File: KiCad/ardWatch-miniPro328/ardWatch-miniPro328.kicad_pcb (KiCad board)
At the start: 2 copper layers, 84.5 x 65.4 mm, 7 parts, among them J1 2-pin_power_input_header, U1 Arduino_Mini_Pro, U2 KY-040_Rotary_Encoder, U3 ST7735_1.8"_TFT_128x160, U4 DS3231_RTC_module

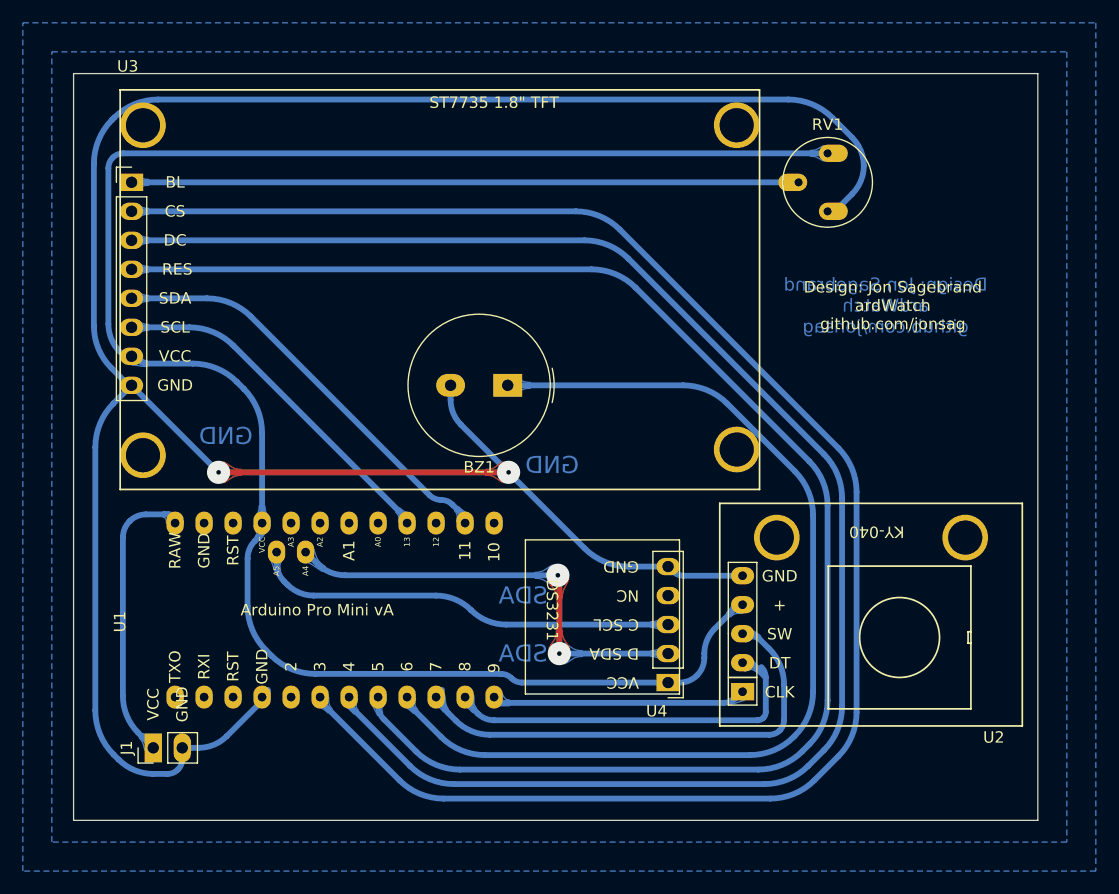
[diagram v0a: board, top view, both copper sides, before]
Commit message: revised pcb
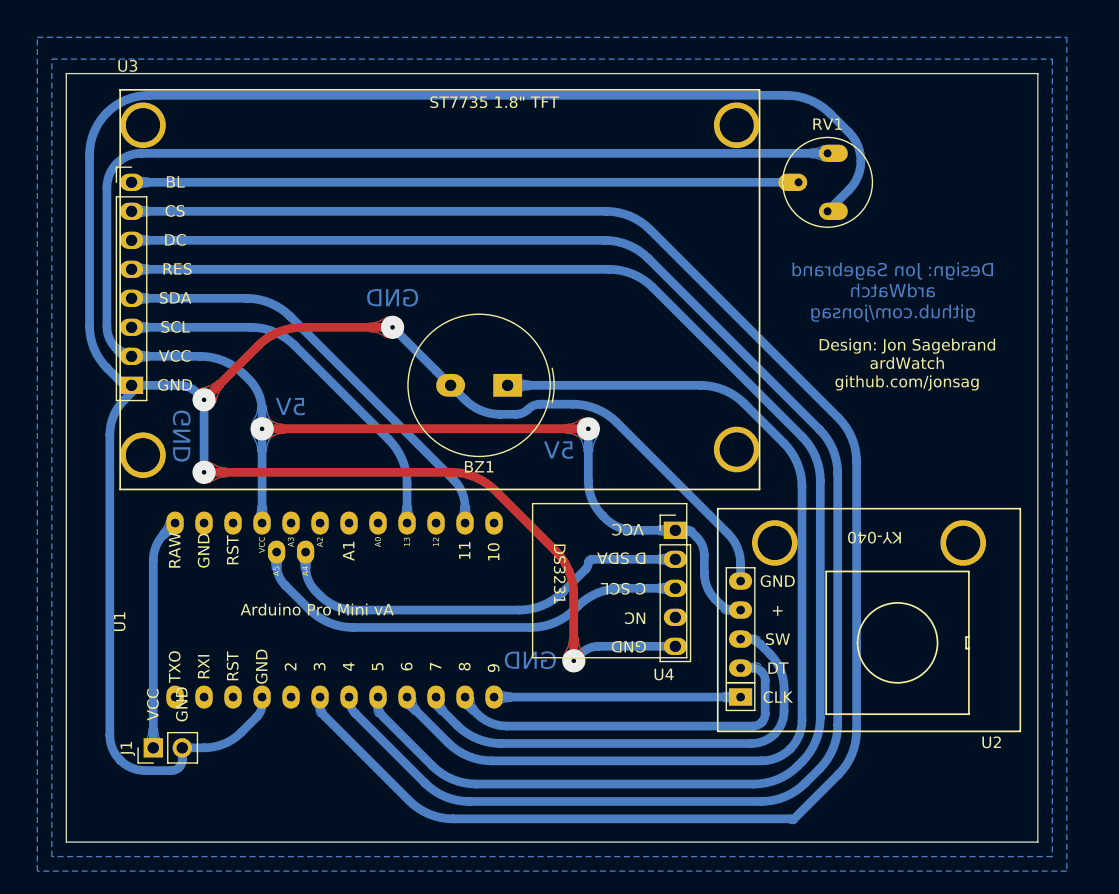
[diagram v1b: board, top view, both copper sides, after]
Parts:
- J1: footprint My_Headers:2-pin_power_input_header_larger_pads -> My_Headers:2-pin_power_input_header
- moved U4 3.24 mm to (127.6, 99.1)
- moved U2 0.50 mm to (133.3, 103.5)
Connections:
- U3 pad 1: Net-(RV1-Pad2) -> GND
- U3 pad 2: Net-(U1-Pad6) -> +5V
- U3 pad 3: Net-(U1-Pad7) -> Net-(U1-Pad21)
- U3 pad 4: Net-(U1-Pad8) -> Net-(U1-Pad23)
- U3 pad 5: Net-(U1-Pad23) -> Net-(U1-Pad8)
- U3 pad 6: Net-(U1-Pad21) -> Net-(U1-Pad7)
- U3 pad 7: +5V -> Net-(U1-Pad6)
- U3 pad 8: GND -> Net-(RV1-Pad2)
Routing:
- net GND: track 221.5 -> 276.2 mm, vias 2 -> 4
- net VCC: track 25.8 -> 20.3 mm
- net Net-(U1-Pad6): track 148.3 -> 153.1 mm
- net Net-(U1-Pad7): track 140.7 -> 144.1 mm
- net Net-(U1-Pad21): track 30.7 -> 34.1 mm
- net SCL: track 37.4 -> 39.4 mm
- net Net-(U1-Pad8): track 133.2 -> 135.1 mm
- net SDA: track 39.2 -> 37.4 mm, vias 2 -> 0
- net Net-(U1-Pad23): track 37.2 -> 38.6 mm
- net +5V: track 158.7 -> 157.5 mm, vias 0 -> 2
- net Net-(BZ1-Pad1): track 88.5 -> 89.6 mm
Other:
- board size 84.5 x 65.4 mm -> 85.1 x 67.3 mm
- board text added: "5V"
- board text removed: "SDA"
